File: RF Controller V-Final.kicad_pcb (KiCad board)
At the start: 2 copper layers, 132 x 67.5 mm, 37 parts, among them J2 J_OLED, J3 BAT+, J4 BAT-, SW1 EG1218, U3 NRF24L01, U5 AP2112K-3.3, U7 Pitch/Roll, U8 TPS542025DDCR, U9 Throttle/Yaw

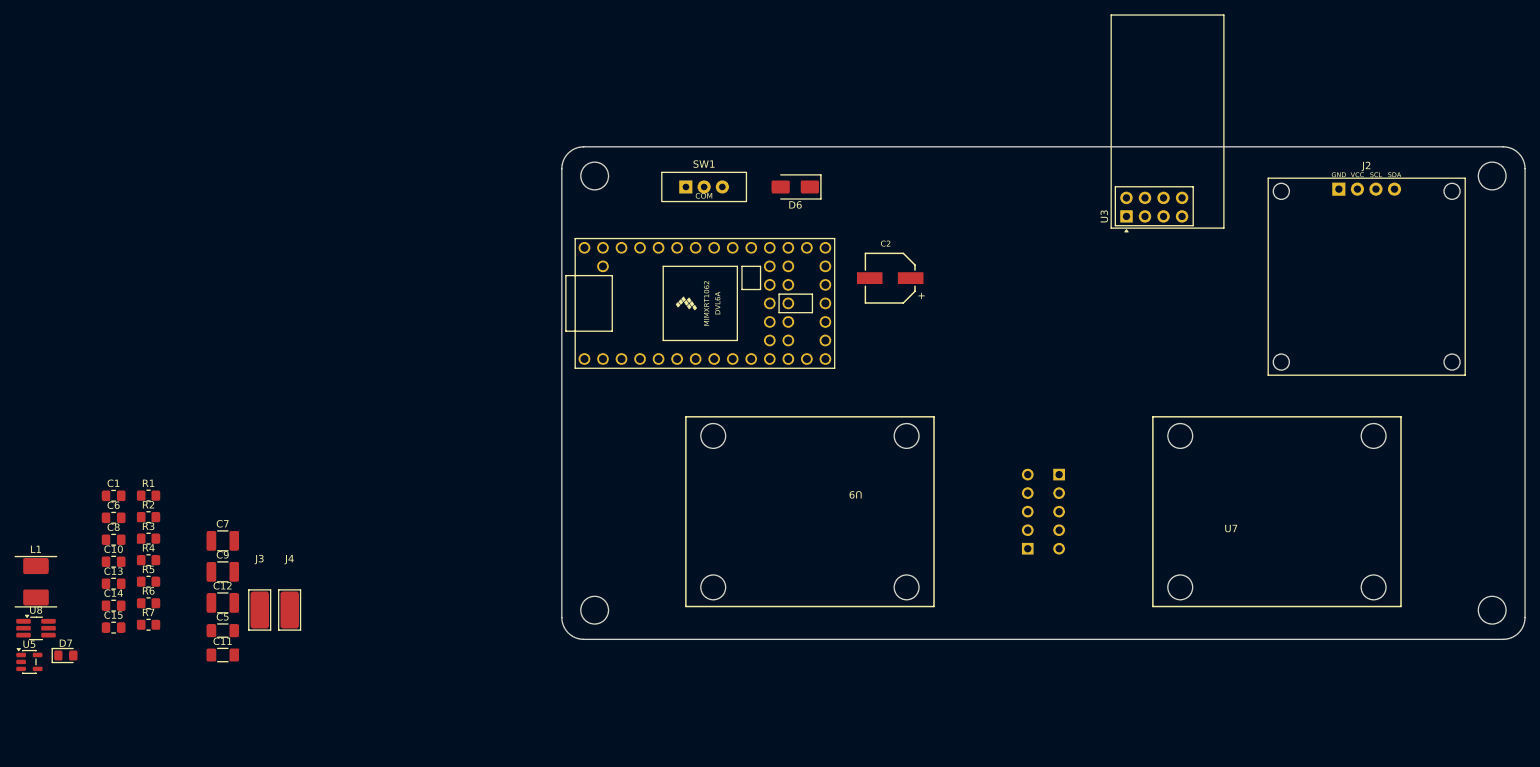
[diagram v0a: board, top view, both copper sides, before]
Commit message: Component layout V1
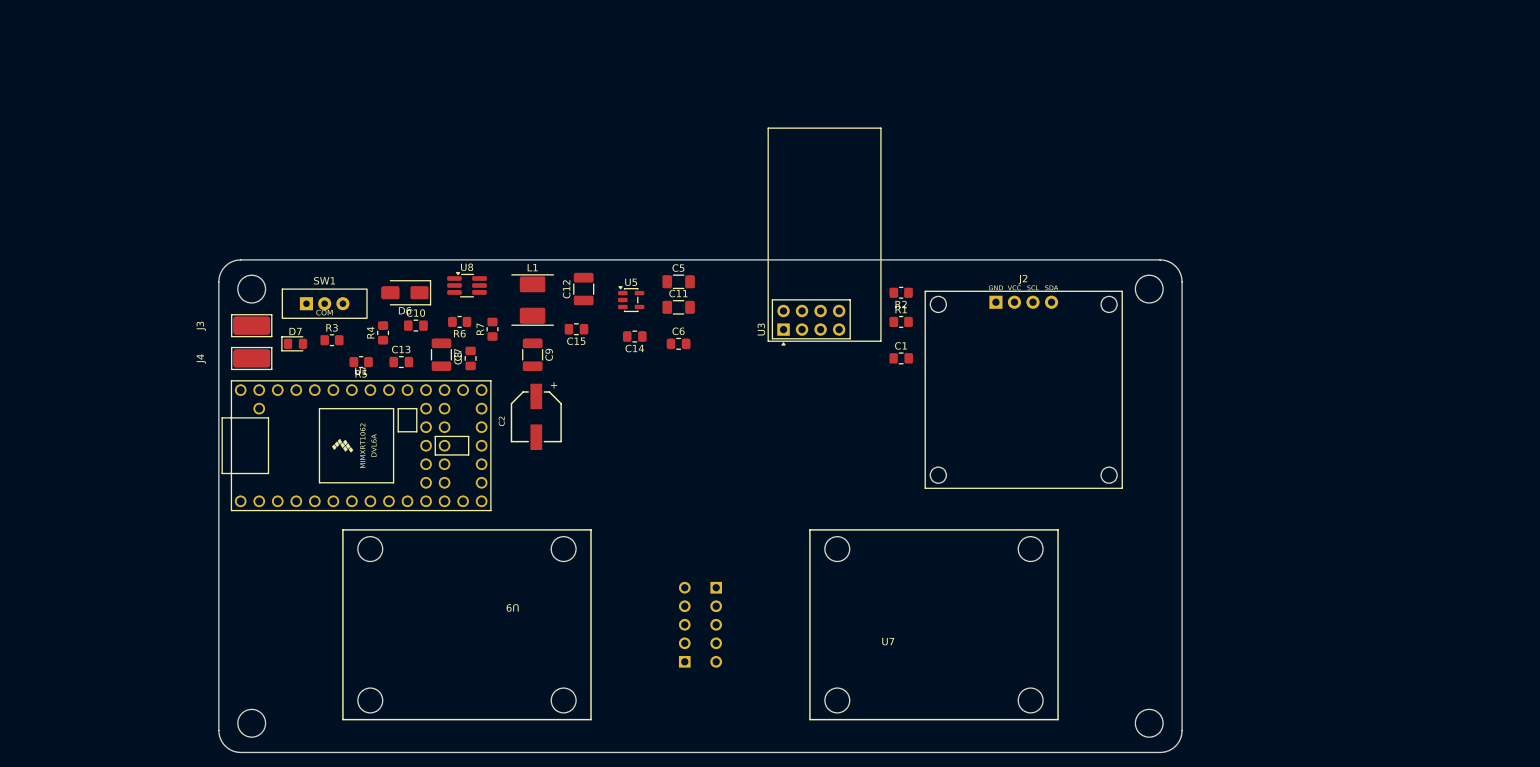
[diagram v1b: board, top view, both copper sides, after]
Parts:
- removed ?: , teensy:Teensy40
- added U1: Teensy4.0, teensy:Teensy40, F.Cu at (101.5, 93.5)
- C11: value 22u -> 10u
- C12: value 10u -> 22u
- D7: value APT2012LZGCK -> (none)
- SW1: value EG1218 -> (none)
- U5: value AP2112K-3.3 -> (none)
- U8: value TPS542025DDCR -> (none)
- moved C1 109.6 mm to (175.5, 81.5)
- moved R2 107.6 mm to (175.5, 72.5), turned to 180 degrees
- moved R1 105.9 mm to (175.5, 76.5)
- moved U5 96.2 mm to (138.5, 73.5)
- moved C6 81.0 mm to (145.0, 79.5)
- moved C14 80.4 mm to (139.0, 78.5), turned to 180 degrees
- moved C5 78.7 mm to (145.0, 71.0)
- moved C11 78.6 mm to (145.0, 74.5)
- moved L1 78.3 mm to (125.0, 73.5)
- moved U8 75.5 mm to (116.0, 71.5)
- moved C15 75.5 mm to (131.0, 77.5), turned to 180 degrees
- moved C12 65.5 mm to (132.0, 72.0), turned to 90 degrees
- moved R7 62.1 mm to (119.5, 77.5), turned to 90 degrees
- moved R6 57.5 mm to (115.0, 76.5), turned to 180 degrees
- moved D6 55.4 mm to (107.5, 72.5)
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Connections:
- net Net-(U8-SW) renamed /BUCK_SW
- C11 pad 1: /5V_IN -> /3.3V_OUT
- C12 pad 1: /3.3V_OUT -> /5V_IN
- SW1 pad 1: unconnected-(SW1-A-Pad1) -> /VBAT
- SW1 pad 3: /VBAT -> unconnected-(SW1-C-Pad3)
